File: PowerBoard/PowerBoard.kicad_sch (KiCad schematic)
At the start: 21 parts, among them J1 Conn_02x02_Odd_Even, J2 Conn_02x02_Odd_Even, J3 Conn_02x02_Odd_Even, J4 Conn_02x02_Odd_Even, U1 LM3150MH

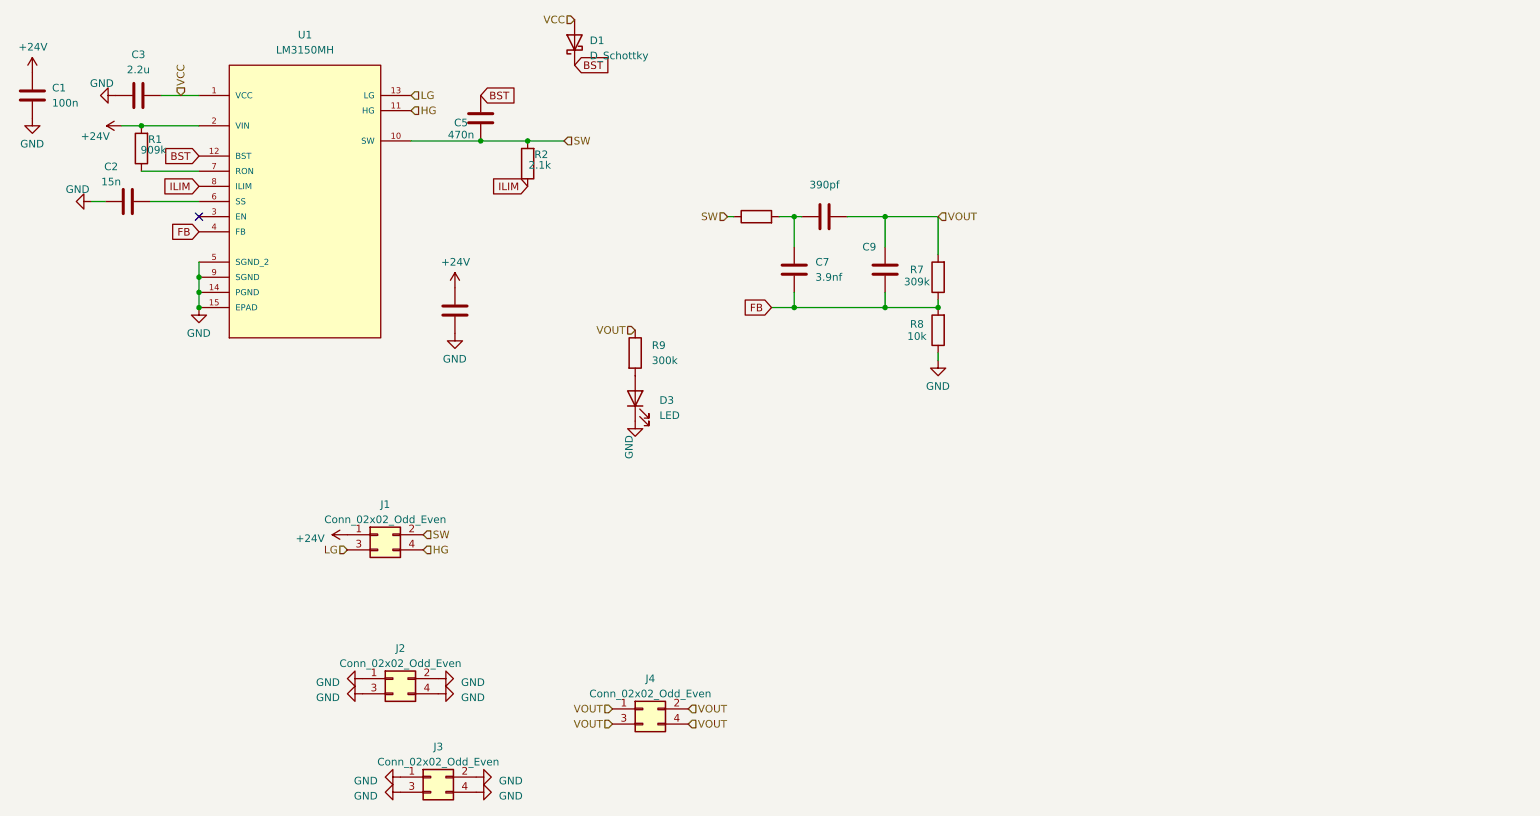
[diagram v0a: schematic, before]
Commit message: 布局
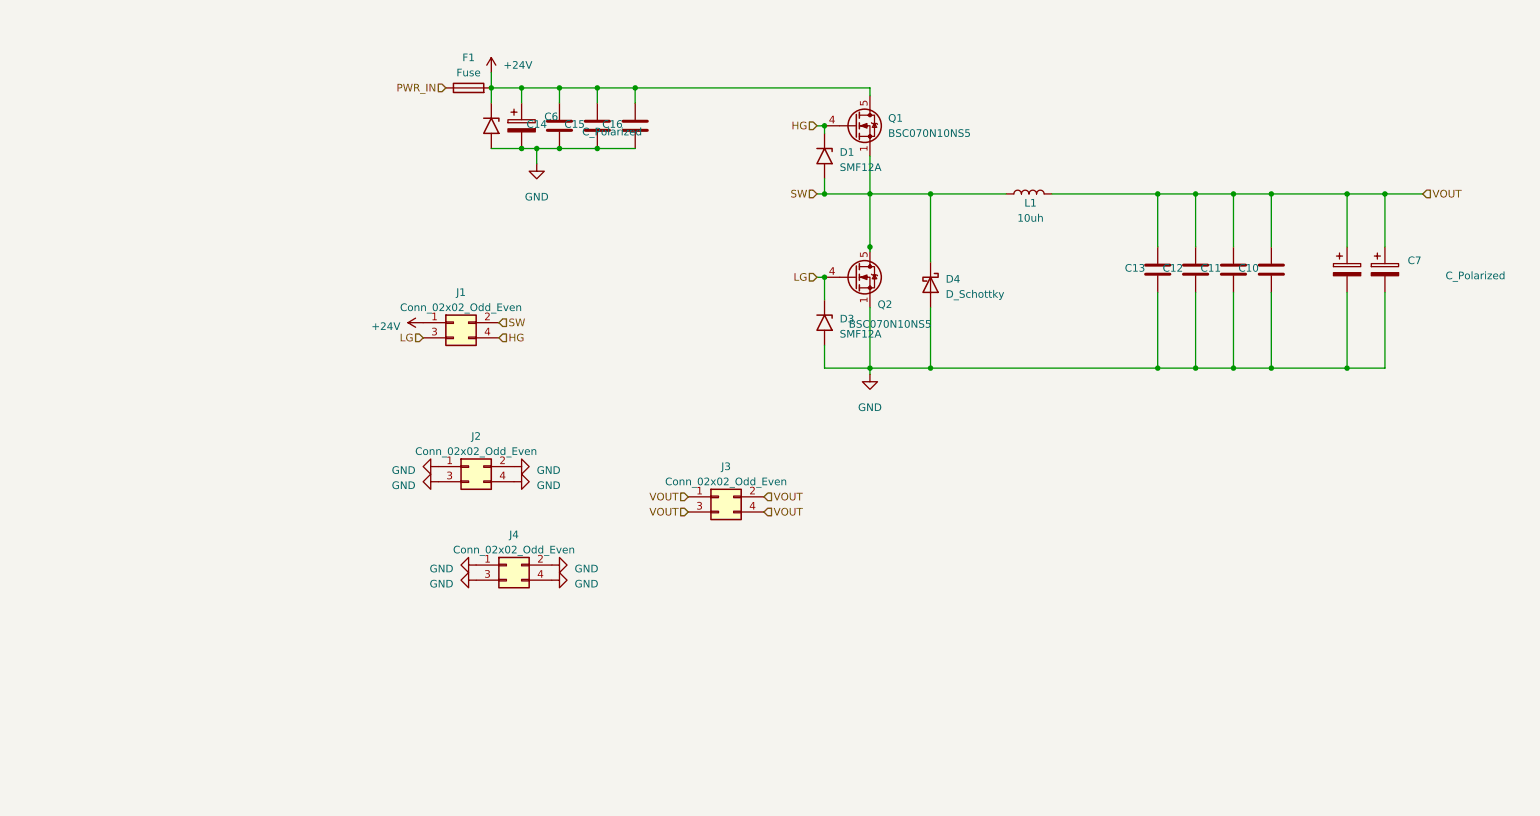
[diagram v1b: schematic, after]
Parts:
- removed C1: 100n, Capacitor_SMD:C_0603_1608Metric, symbol Device:C
- removed C2: 15n, Capacitor_SMD:C_0603_1608Metric, symbol Device:C
- removed C3: 2.2u, Capacitor_SMD:C_0603_1608Metric, symbol Device:C
- removed C4: 22u, Capacitor_SMD:C_0603_1608Metric, symbol Device:C
- removed C5: 470n, Capacitor_SMD:C_0603_1608Metric, symbol Device:C
- removed C7: 3.9nf, Capacitor_SMD:C_0603_1608Metric, symbol Device:C
- removed C8: 390pf, Capacitor_SMD:C_0603_1608Metric, symbol Device:C
- removed C9: ~, Capacitor_SMD:C_0603_1608Metric, symbol Device:C
- removed D1: D_Schottky, Diode_SMD:D_SMF, symbol Device:D_Schottky
- removed D3: LED, LED_SMD:LED_0603_1608Metric, symbol Device:LED
- removed R1: 909k, Resistor_SMD:R_0603_1608Metric, symbol Device:R
- removed R2: 2.1k, Resistor_SMD:R_0603_1608Metric, symbol Device:R
- removed R5: 8.06M, Resistor_SMD:R_0603_1608Metric, symbol Device:R
- removed R7: 309k, Resistor_SMD:R_0603_1608Metric, symbol Device:R
- removed R8: 10k, Resistor_SMD:R_0603_1608Metric, symbol Device:R
- removed R9: 300k, Resistor_SMD:R_0603_1608Metric, symbol Device:R
- removed U1: LM3150MH, Package_SO:HTSSOP-14-1EP_4.4x5mm_P0.65mm_EP3.4x5mm_Mask3x3.1mm, symbol 0_RM2023:LM3150MH
- added C10, C11, C12, C13, C14, C15, C16: 100u, Capacitor_SMD:C_1206_3216Metric, symbol Device:C
- added C4, C6, C7: C_Polarized, Capacitor_SMD:CP_Elec_10x10, symbol Device:C_Polarized
- added D1, D3: SMF12A, Diode_SMD:D_SMF, symbol Diode:SMF12A
- added D2: SM6T30A, Diode_SMD:D_SMC, symbol Diode:SM6T30A
- added D4: D_Schottky, Diode_SMD:D_PowerDI-5, symbol Device:D_Schottky
- added F1: Fuse, Fuse:Fuseholder_Littelfuse_Nano2_157x, symbol Device:Fuse
- added L1: 10uh, 0_RM2023:Inductor_RM6, symbol Device:L
- added Q1, Q2: BSC070N10NS5, Package_TO_SOT_SMD:TDSON-8-1, symbol Transistor_FET:BSC070N10NS5
- J1, J2, J3, J4: footprint 0_RM2023:conn_2x02_2.54 -> Connector_PinHeader_2.54mm:PinHeader_2x02_P2.54mm_Vertical_SMD
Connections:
- net +24V: now also C14.2, C15.2, C16.2, C6.1, D2.1 (A1), F1.2, Q1.5 (D)
- net GND: now also J4.1 (Pin_1), J4.2 (Pin_2), J4.3 (Pin_3), J4.4 (Pin_4), C10.1, C11.1, C12.1, C13.1, C14.1, C15.1, C16.1, C4.2, C6.2, C7.2, D2.2 (A2), D3.2 (A2), D4.2 (A), Q2.1 (S), Q2.2 (S), Q2.3 (S); no longer J3.1 (Pin_1), J3.2 (Pin_2), J3.3 (Pin_3), J3.4 (Pin_4)
- net HG: now also D1.1 (A1), Q1.4 (G)
- net LG: now also D3.1 (A1), Q2.4 (G)
- net SW: now also D1.2 (A2), D4.1 (K), L1.1, Q1.1 (S), Q1.2 (S), Q1.3 (S), Q2.5 (D)
- net VOUT: now also J3.1 (Pin_1), J3.2 (Pin_2), J3.3 (Pin_3), J3.4 (Pin_4), C10.2, C11.2, C12.2, C13.2, C4.1, C7.1, L1.2; no longer J4.1 (Pin_1), J4.2 (Pin_2), J4.3 (Pin_3), J4.4 (Pin_4)
- new net PWR_IN: F1.1
- no-connect marks 1 -> 0
